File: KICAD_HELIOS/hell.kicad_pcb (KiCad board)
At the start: 4 copper layers, 109 x 86 mm, 171 parts, among them J101 NC3FAAH, J102 NC3MAAH, J103 ecran, J104 Conn_ST_STDC14, J105 Conn_01x02, SW101 SW_Push, SW102 SW_Push, SW103 SW_Push, U101 R-78B5.0-2.0, U102 AZ1117CH2-3.3TRG1, U103 MAX485E, U104 STM32F103C6Tx, U1101 LM3404MA, U1102 LM3404MA, U1103 LM3404MA, U201 LM3404MA, U202 LM3404MA, U203 LM3404MA

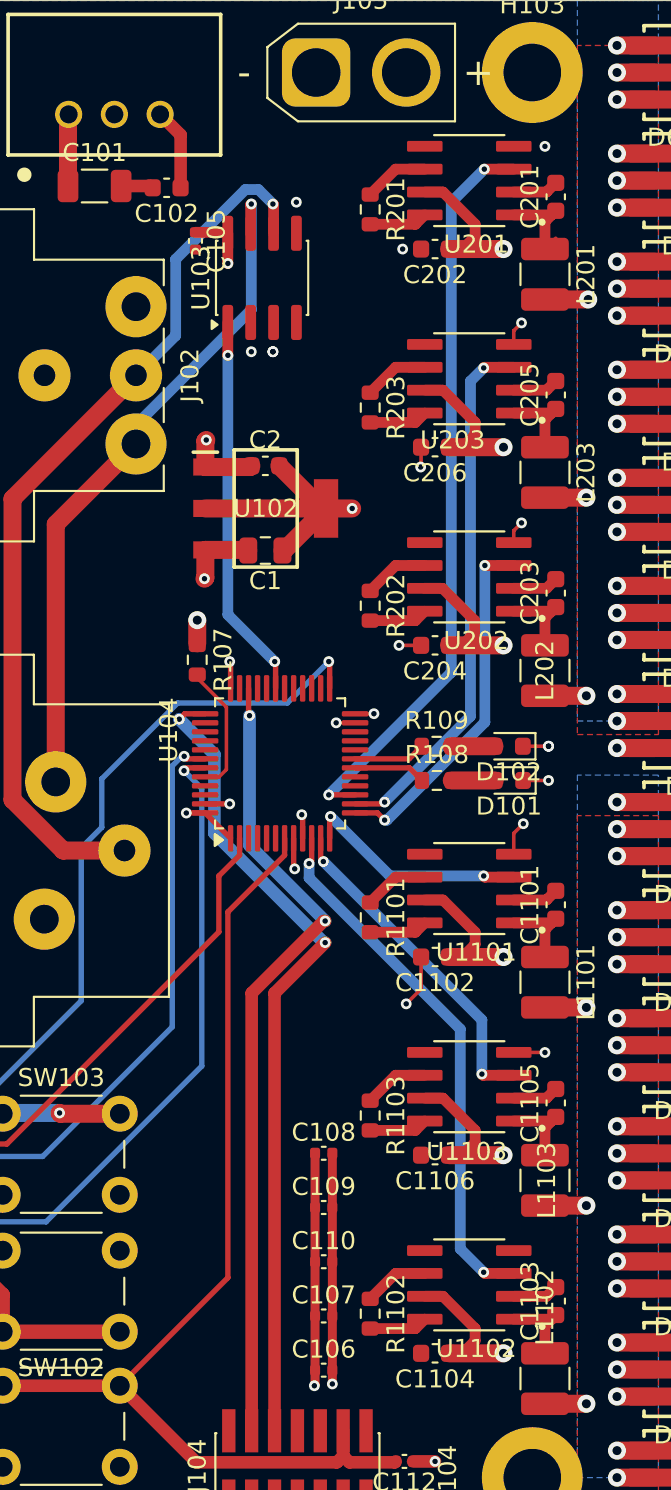
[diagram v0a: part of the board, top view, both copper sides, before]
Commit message: pcb
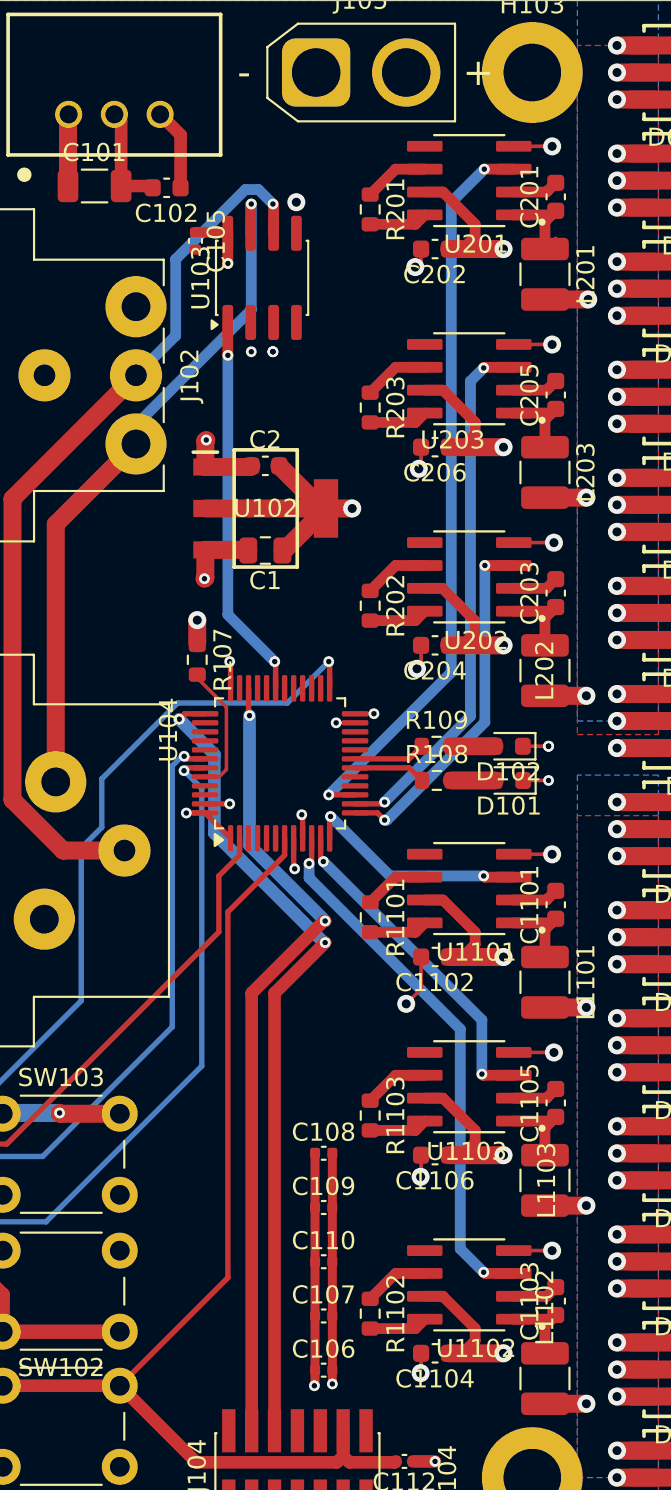
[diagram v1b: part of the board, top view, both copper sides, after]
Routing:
- net GND: track 177.6 -> 192.2 mm, vias 69 -> 72
